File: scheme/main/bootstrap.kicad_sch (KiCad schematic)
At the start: 7 parts, among them U1 B2415LS-1WR3

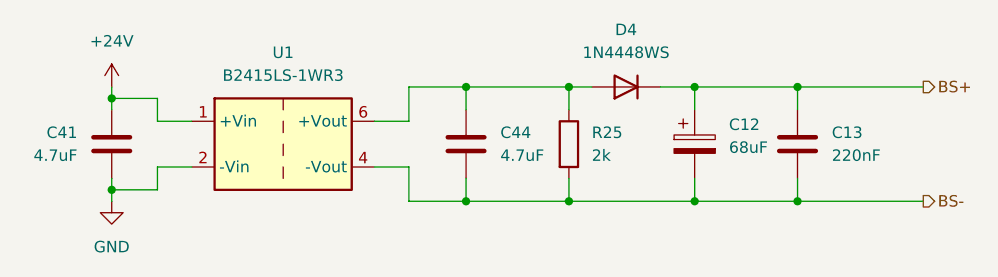
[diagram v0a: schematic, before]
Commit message: power scheme
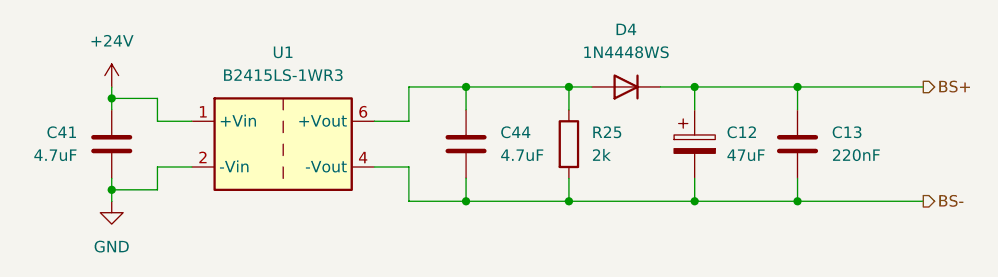
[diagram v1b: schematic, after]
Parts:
- C12: value 68uF -> 47uF; footprint Capacitor_SMD:C_Elec_6.3x7.7 -> Capacitor_SMD:C_Elec_5x5.8
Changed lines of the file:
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@@
 		(shape output)
 		(at 156.21 86.36 0)
+		(fields_autoplaced yes)
 		(effects
 			(font
@@
 		(shape output)
 		(at 156.21 73.66 0)
+		(fields_autoplaced yes)
 		(effects
 			(font
@@
 		(dnp no)
 		(property "Reference" "C12"
-			(at 134.62 77.8509 0)
+			(at 134.366 78.74 0)
 			(effects
 				(font
@@
 			)
 		)
-		(property "Value" "68uF"
-			(at 134.62 80.3909 0)
+		(property "Value" "47uF"
+			(at 134.366 81.28 0)
 			(effects
 				(font
@@
 			)
 		)
-		(property "Footprint" "Capacitor_SMD:C_Elec_6.3x7.7"
+		(property "Footprint" "Capacitor_SMD:C_Elec_5x5.8"
 			(at 131.7752 83.82 0)
 			(effects
@@
 			)
 		)
-		(property "Datasheet" "https://doc.platan.ru/pdf/datasheets/panasonic/FK_V.pdf"
+		(property "Datasheet" "https://www.platan.ru/cgi-bin/qwery.pl/id=2015355001"
 			(at 130.81 80.01 0)
 			(effects
